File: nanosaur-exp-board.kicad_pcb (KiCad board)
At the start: 2 copper layers, 80 x 20 mm, 13 parts, among them J1 jetson_nano, J2 Screw_Terminal_01x02, J3 Conn_oled_right, J4 Conn_oled_left, J5 Conn_motors, J6 Conn_01x03, SW1 SW_SPDT

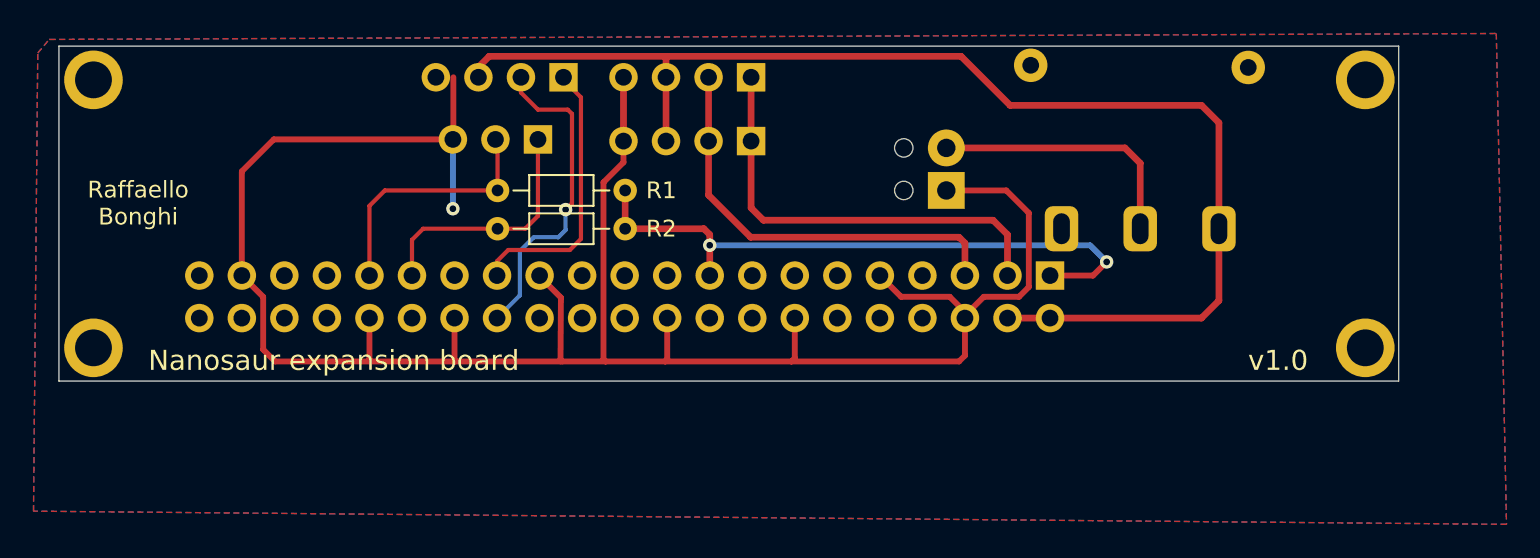
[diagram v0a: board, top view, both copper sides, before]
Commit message: Improve sch and pcb
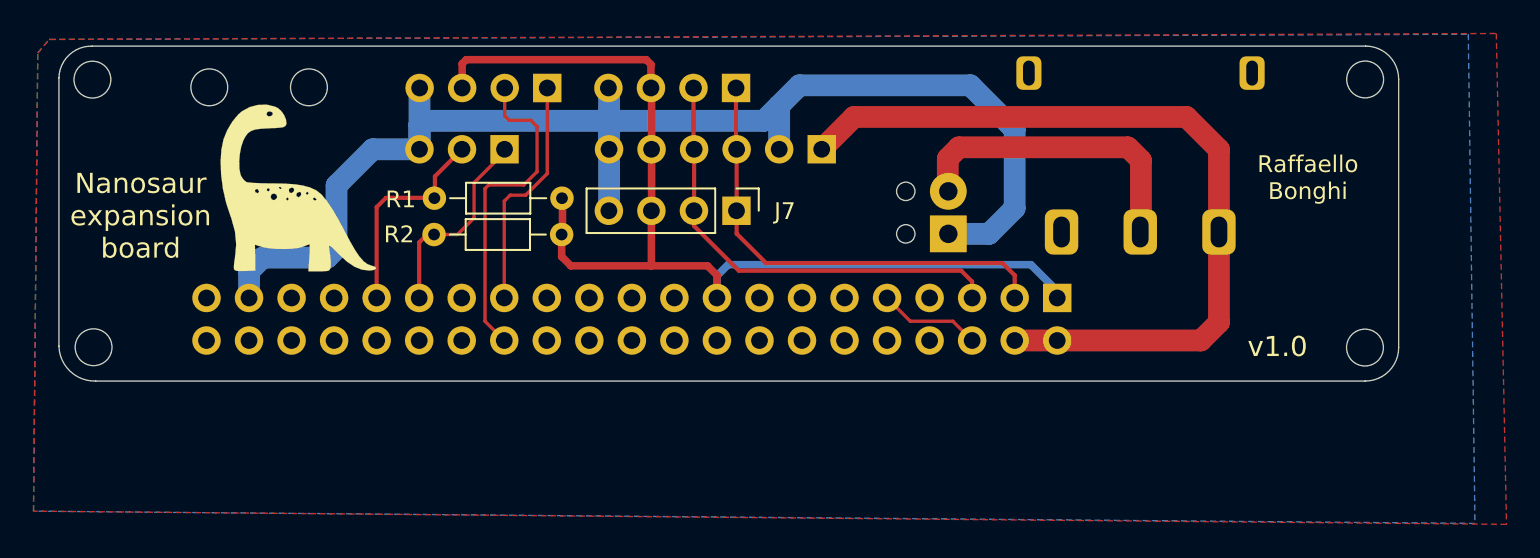
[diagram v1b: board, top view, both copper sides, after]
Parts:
- added G***: LOGO, nanosaur:nanosaur_logo, F.Cu at (121.2, 91.8)
- added H5: MountingHole, MountingHole:MountingHole_2.2mm_M2, F.Cu at (116.0, 85.8)
- added H6: MountingHole, MountingHole:MountingHole_2.2mm_M2, F.Cu at (122.0, 85.8)
- added J7: Conn_01x04, Connector_PinHeader_2.54mm:PinHeader_1x04_P2.54mm_Vertical, F.Cu at (147.5, 93.2)
- H1, H2, H3, H4: footprint MountingHole:MountingHole_2.2mm_M2_ISO7380_Pad -> MountingHole:MountingHole_2.2mm_M2
- J3: value Conn_oled_right -> Conn_01x04
- J4: value Conn_oled_left -> Conn_01x04
- J5: value Conn_motors -> Conn_01x06; footprint Connector_PinHeader_2.54mm:PinHeader_1x04_P2.54mm_Vertical -> Connector_PinHeader_2.54mm:PinHeader_1x06_P2.54mm_Vertical
- moved J5 4.25 mm to (152.6, 89.5)
- moved R2 3.81 mm to (137.1, 94.6)
- moved R1 3.80 mm to (137.1, 92.4)
- moved J2 2.59 mm to (160.1, 94.5)
- moved J6 2.08 mm to (133.6, 89.5)
- moved J1 1.41 mm to (166.6, 98.4)
- moved J3 1.16 mm to (136.2, 85.8)
- moved J4 1.10 mm to (147.5, 85.8)
- moved SW1 0.20 mm to (171.6, 94.4)
- moved H1 0.06 mm to (109.0, 85.3)
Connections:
- J1 pad 10: Net-(J1-Pad10) -> (no net)
- J1 pad 11: Net-(J1-Pad11) -> (no net)
- J1 pad 12: Net-(J1-Pad12) -> (no net)
- J1 pad 13: Net-(J1-Pad13) -> (no net)
- J1 pad 15: Net-(J1-Pad15) -> (no net)
- J1 pad 16: Net-(J1-Pad16) -> (no net)
- J1 pad 18: Net-(J1-Pad18) -> (no net)
- J1 pad 19: Net-(J1-Pad19) -> (no net)
- J1 pad 21: Net-(J1-Pad21) -> (no net)
- J1 pad 22: Net-(J1-Pad22) -> (no net)
- J1 pad 23: Net-(J1-Pad23) -> (no net)
- J1 pad 24: Net-(J1-Pad24) -> (no net)
- J1 pad 26: Net-(J1-Pad26) -> (no net)
- J1 pad 29: Net-(J1-Pad29) -> (no net)
- J1 pad 32: Net-(J1-Pad32) -> (no net)
- J1 pad 35: Net-(J1-Pad35) -> (no net)
- J1 pad 36: Net-(J1-Pad36) -> (no net)
- J1 pad 37: Net-(J1-Pad37) -> (no net)
- J1 pad 38: Net-(J1-Pad38) -> (no net)
- J1 pad 40: Net-(J1-Pad40) -> (no net)
- J1 pad 7: Net-(J1-Pad7) -> (no net)
- J1 pad 8: Net-(J1-Pad8) -> (no net)
- J3 pad 3: VCC -> +3V3
- J4 pad 3: VCC -> +3V3
- J5 pad 1: Net-(J1-Pad3) -> VCC
- J5 pad 2: Net-(J1-Pad5) -> GND
- J5 pad 3: VCC -> Net-(J1-Pad3)
- J5 pad 4: GND -> Net-(J1-Pad5)
- SW1 pad 3: Net-(SW1-Pad3) -> (no net)
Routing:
- net GND: track 131.6 -> 88.2 mm, vias 1 -> 0
- net VCC: track 76.2 -> 48.3 mm
- net +3V3: track 37.8 -> 63.1 mm, vias 2 -> 0
- net Net-(J2-Pad2): track 15.0 -> 17.7 mm
- net Net-(J1-Pad31): track 15.0 -> 12.3 mm
- net Net-(J1-Pad33): track 15.3 -> 12.7 mm
- net Net-(J1-Pad27): track 16.5 -> 14.5 mm
- net Net-(J1-Pad5): track 25.5 -> 27.2 mm
- net Net-(J1-Pad3): track 26.2 -> 27.7 mm
- net Net-(J1-Pad28): track 19.4 -> 19.6 mm, vias 1 -> 0
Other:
- outline, holes or cut-outs redrawn
- net class 3.3 line added: clearance 0.2, trace_width 0.45, via_dia 0.8, via_drill 0.4
- net class POWER: trace_width 0.35 -> 1.3
